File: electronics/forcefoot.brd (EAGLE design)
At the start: 55 x 45.2 mm, 62 parts

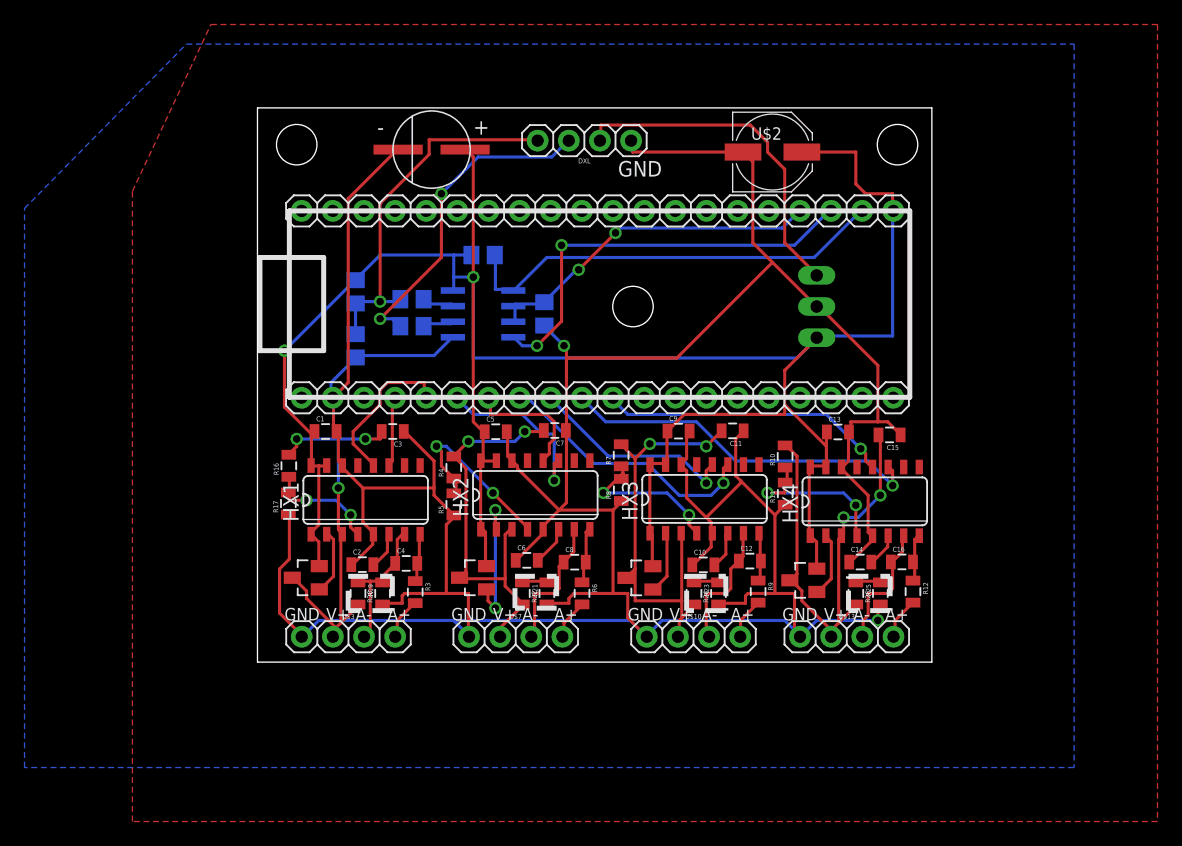
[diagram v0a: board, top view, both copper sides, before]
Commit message: Tweaking for v2
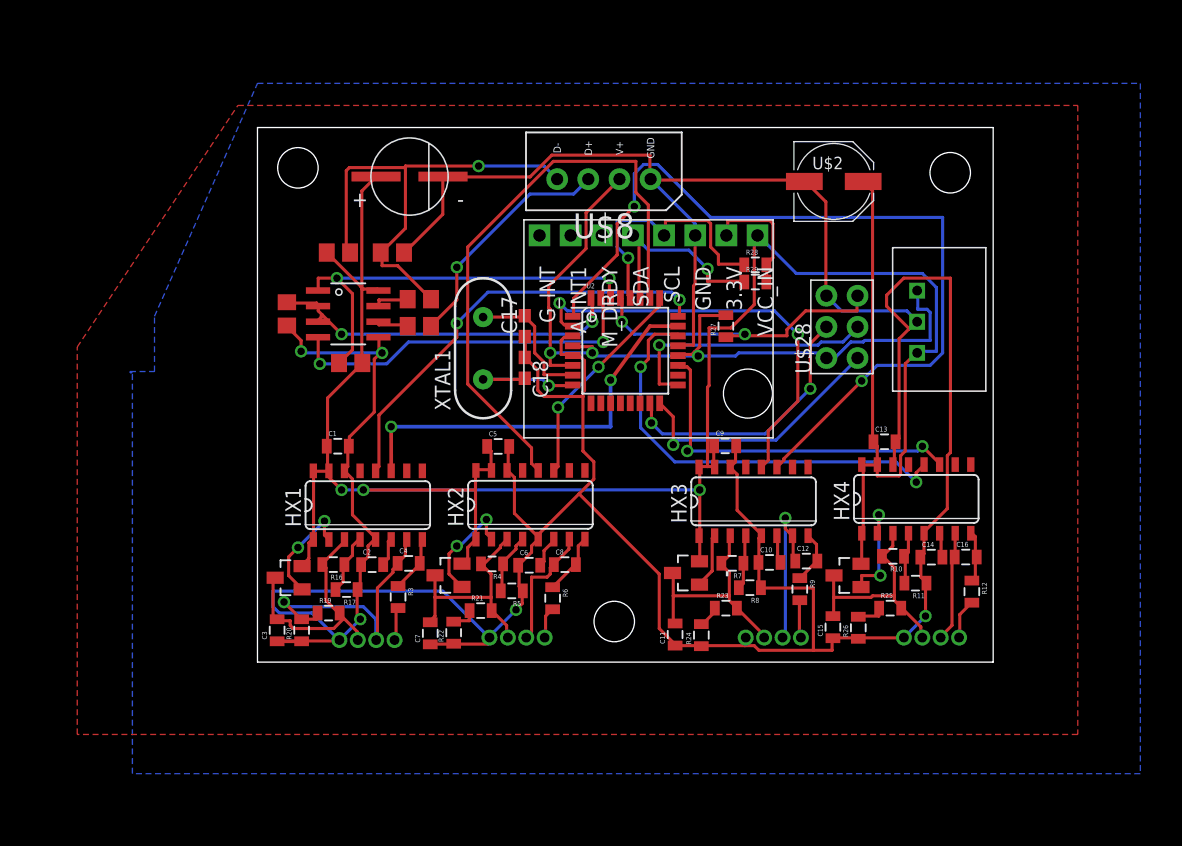
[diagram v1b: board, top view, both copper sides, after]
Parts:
- removed DXL: CONNEC_1X04, rhoban:CONNEC_1X04
- removed IC1: (no value), SparkFun-PowerIC:TO-220-ALT
- removed MAPLE_MINI: MAPLE_MINI, rhoban:CONNEC_2X20
- removed U$15: (no value), SparkFun-Electromechanical:STAND-OFF
- added C17, C18: 22, rhoban:C0603
- added R27: 10k, SparkFun-Passives:0805
- added R28, R29: 3K, SparkFun-Passives:0805
- added U$11, U$14: (no value), SparkFun-Electromechanical:STAND-OFF
- added U$17: GY-85, rhoban:GY-85
- added U$28: CONNEC_2X03, rhoban:CONNEC_2X03
- added U$5: REG_5V, rhoban:TRACOPOWER
- added U$8: CONNEC_1X04_485, rhoban:CONNEC_485
- added U2: ATMEGA168, SparkFun-DigitalIC:TQFP32-08
- added XTAL1: (no value), rhoban:HC49US
- U$10, U$13, U$3, U$7: value CONNEC_1X04 -> CONNEC_1X041.5; device rhoban:CONNEC_1X04 -> rhoban:4P1.5
- moved U$16 45.2 mm to (29.1, 3.11)
- moved R1 21.0 mm to (2.40, 28.2), flipped to the top
- moved C7 19.4 mm to (14.1, 2.15), turned to 90 degrees
- moved C3 18.8 mm to (1.60, 2.40), turned to 90 degrees
- moved C11 17.3 mm to (34.1, 2.05), turned to 90 degrees
- moved C15 16.3 mm to (46.9, 2.65), turned to 90 degrees
- moved R13 13.9 mm to (7.60, 24.2), flipped to the top
- moved R8 13.2 mm to (40.2, 5.87), turned to 180 degrees
- moved R11 12.9 mm to (53.7, 6.24), turned to 180 degrees
- moved R7 12.6 mm to (38.7, 7.86), turned to 180 degrees
- moved R10 12.0 mm to (51.8, 8.43), turned to 180 degrees
- moved MAX485 11.0 mm to (7.40, 28.2), flipped to the top
- moved R16 8.84 mm to (6.19, 7.76), turned to 180 degrees
- moved R5 8.49 mm to (20.7, 5.61), turned to 180 degrees
- moved R17 8.47 mm to (7.26, 5.72), turned to 180 degrees
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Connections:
- new net 3.3: R28.2, R29.2, U$17.3.3
- new net IMU_SCL: R28.1, U$17.SCL, U2.28
- new net IMU_SDA: R29.1, U$17.SDA, U2.27
- new net MISO: U$28.1, U2.16
- new net MOSI: U$28.4, U2.15
- new net N$19: C17.2, U2.7, XTAL1.2
- new net N$20: C18.2, U2.8, XTAL1.1
- new net RESET: R27.1, U$28.5, U2.29
- new net SCK: U$28.3, U2.17
- net 1A+: now also U$3.P$4; no longer U$3.4
- net 1A-: now also U$3.P$3; no longer U$3.3
- net 2A-: now also U$7.P$3; no longer U$7.3
- net 3A-: now also U$10.P$3; no longer U$10.3
- net 4A-: now also U$13.P$3; no longer U$13.3
- net AVDD$1: now also U$3.P$2; no longer U$3.2
- net AVDD$2: now also U$7.P$2; no longer U$7.2
- net AVDD$3: now also U$10.P$2; no longer U$10.2
- net AVDD$4: now also U$13.P$2; no longer U$13.2
- net DIRECTION: now also U2.32; no longer MAPLE_MINI.X2
- net DOUT1: now also U2.24; no longer MAPLE_MINI.X16
- net DOUT2: now also U2.26; no longer MAPLE_MINI.X18
- net DOUT3: now also U2.2; no longer MAPLE_MINI.X20
- net DOUT4: now also U2.22; no longer MAPLE_MINI.X22
- net GND: now also C17.1, C18.1, U$10.P$1, U$13.P$1, U$17.GND, U$28.6, U$3.P$1, U$5.P$2, U$7.P$1, U$8.GND, U2.21, U2.3, U2.5; no longer DXL.1, IC1.GND, MAPLE_MINI.GND, U$10.1, U$13.1, U$3.1, U$7.1
- net N$4: now also U$7.P$4; no longer U$7.4
- net N$6: now also U$10.P$4; no longer U$10.4
- net N$8: now also U$13.P$4; no longer U$13.4
- net RS+: now also U$8.D+; no longer DXL.3
- net RS-: now also U$8.D-; no longer DXL.4
- net RX: now also U2.30; no longer MAPLE_MINI.X0
- net SCK1: now also U2.23; no longer MAPLE_MINI.X15
- net SCK2: now also U2.25; no longer MAPLE_MINI.X17
- net SCK3: now also U2.1; no longer MAPLE_MINI.X19
- net SCK4: now also U2.19; no longer MAPLE_MINI.X21
- net TX: now also U2.31; no longer MAPLE_MINI.X1
- net VCC: now also U$17.VCC_IN, U$5.P$3; no longer IC1.OUT, MAPLE_MINI.VIN
- net VIN: now also R27.2, U$28.2, U$5.P$1, U$8.V+, U2.20, U2.4, U2.6; no longer DXL.2, IC1.IN
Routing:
- net SCK3: track 22.1 -> 69.4 mm, vias 1 -> 2
- net DOUT2: track 10.4 -> 48.8 mm
- net VIN: track 28.0 -> 65.7 mm, vias 0 -> 3
- net SCK1: track 5.71 -> 33.0 mm, vias 0 -> 2
- net RESET: track 0.00 -> 25.8 mm, vias 0 -> 2
- net DOUT1: track 13.0 -> 35.7 mm, vias 0 -> 2
- net MOSI: track 0.00 -> 22.1 mm, vias 0 -> 2
- net IMU_SCL: track 0.00 -> 21.9 mm, vias 0 -> 1
- net MISO: track 0.00 -> 21.8 mm, vias 0 -> 1
- net SCK: track 0.00 -> 21.6 mm, vias 0 -> 1
- net AVDD$4: track 38.7 -> 18.7 mm, vias 2 -> 0
- net DOUT3: track 17.3 -> 35.2 mm, vias 1 -> 2
- net AVDD$3: track 36.3 -> 18.8 mm, vias 2 -> 0
- net IMU_SDA: track 0.00 -> 16.6 mm, vias 0 -> 1
- net AVDD$2: track 33.0 -> 18.6 mm, vias 2 -> 0
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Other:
- board size 55 x 45.2 mm -> 60 x 43.6 mm
- board text removed: "A+"
- board text removed: "A-"
- board text removed: "GND"
- board text removed: "V+"
